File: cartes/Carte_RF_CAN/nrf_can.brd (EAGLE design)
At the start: 34.2 x 39.4 mm, 13 parts, among them Q1 16MHz

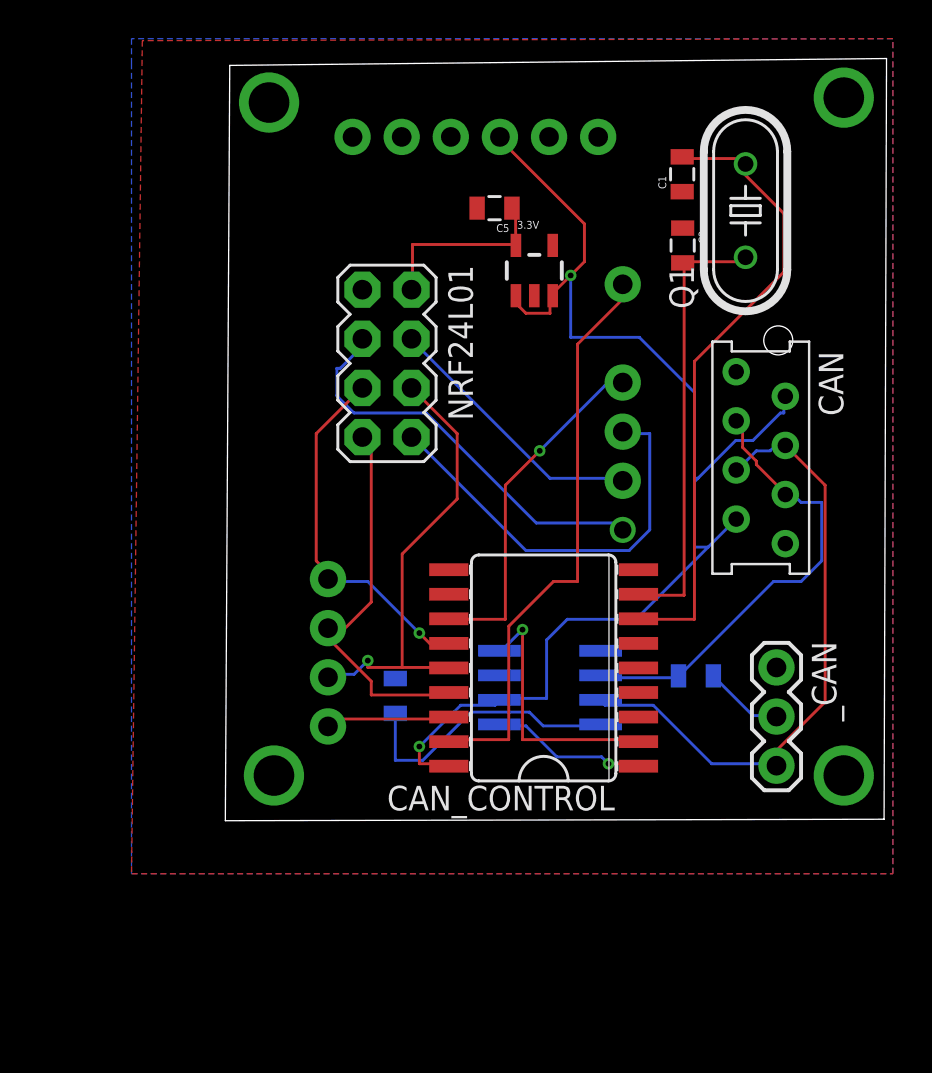
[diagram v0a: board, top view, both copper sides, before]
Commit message: a
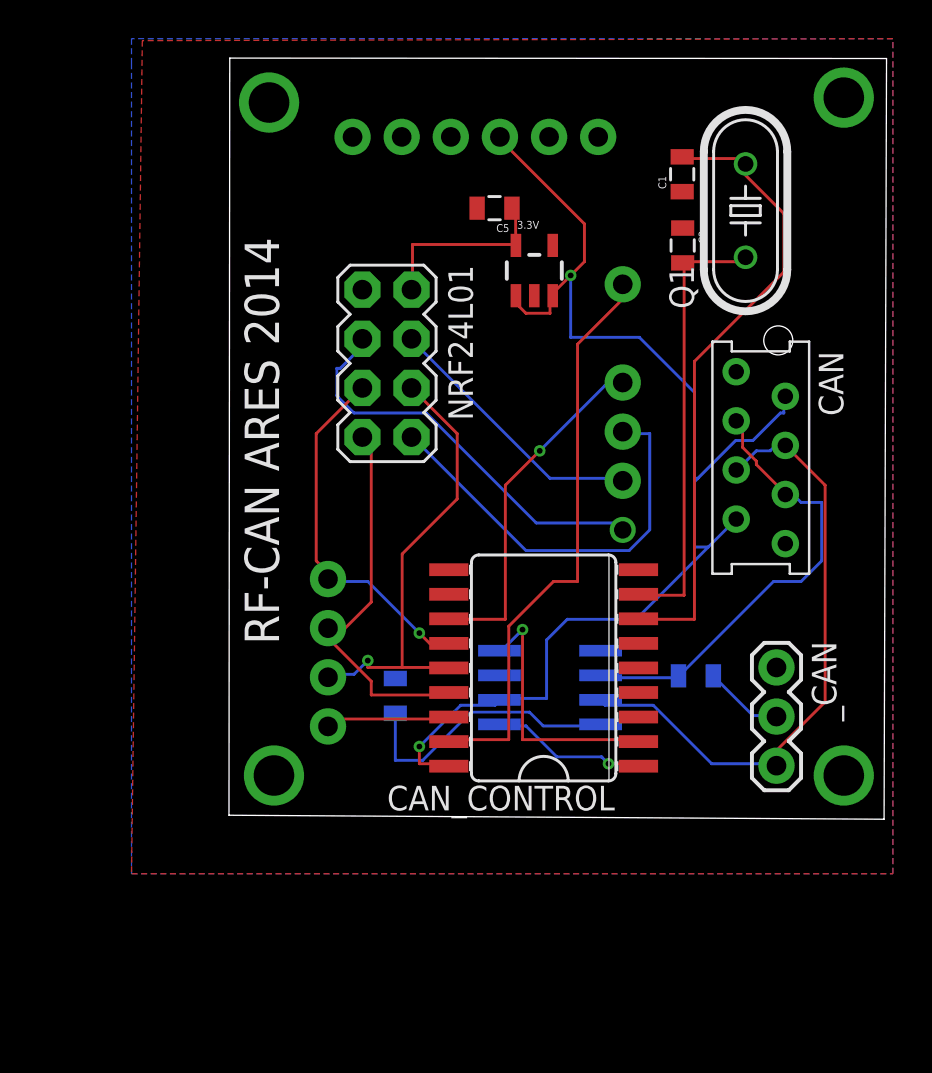
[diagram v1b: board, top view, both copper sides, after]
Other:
- board size 34.2 x 39.4 mm -> 34 x 39.4 mm
- board text added: "/home/showok/.eagle/logo_ares_3.bmp"
- board text added: "RF-CAN ARES 2014"
- board text added: "aaa"
